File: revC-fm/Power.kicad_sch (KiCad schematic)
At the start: 55 parts, among them Q15 MMDT5551-7-F, Q16 MMDT5551-7-F, Q18 IRF7404TRPBF, Q32 MMBT4403WT1G, SW3 USB Charge Inhibit, SW4 High Inhibit, SW5 High USB Inhibit, SW6 Low Inhibit, U18 TPS54226PWPRPWP14_2P31X2P46-L, U19 ADM1176-1ARMZ-R7, U20 ADM1176-1ARMZ-R7, U21 BQ25883RGER

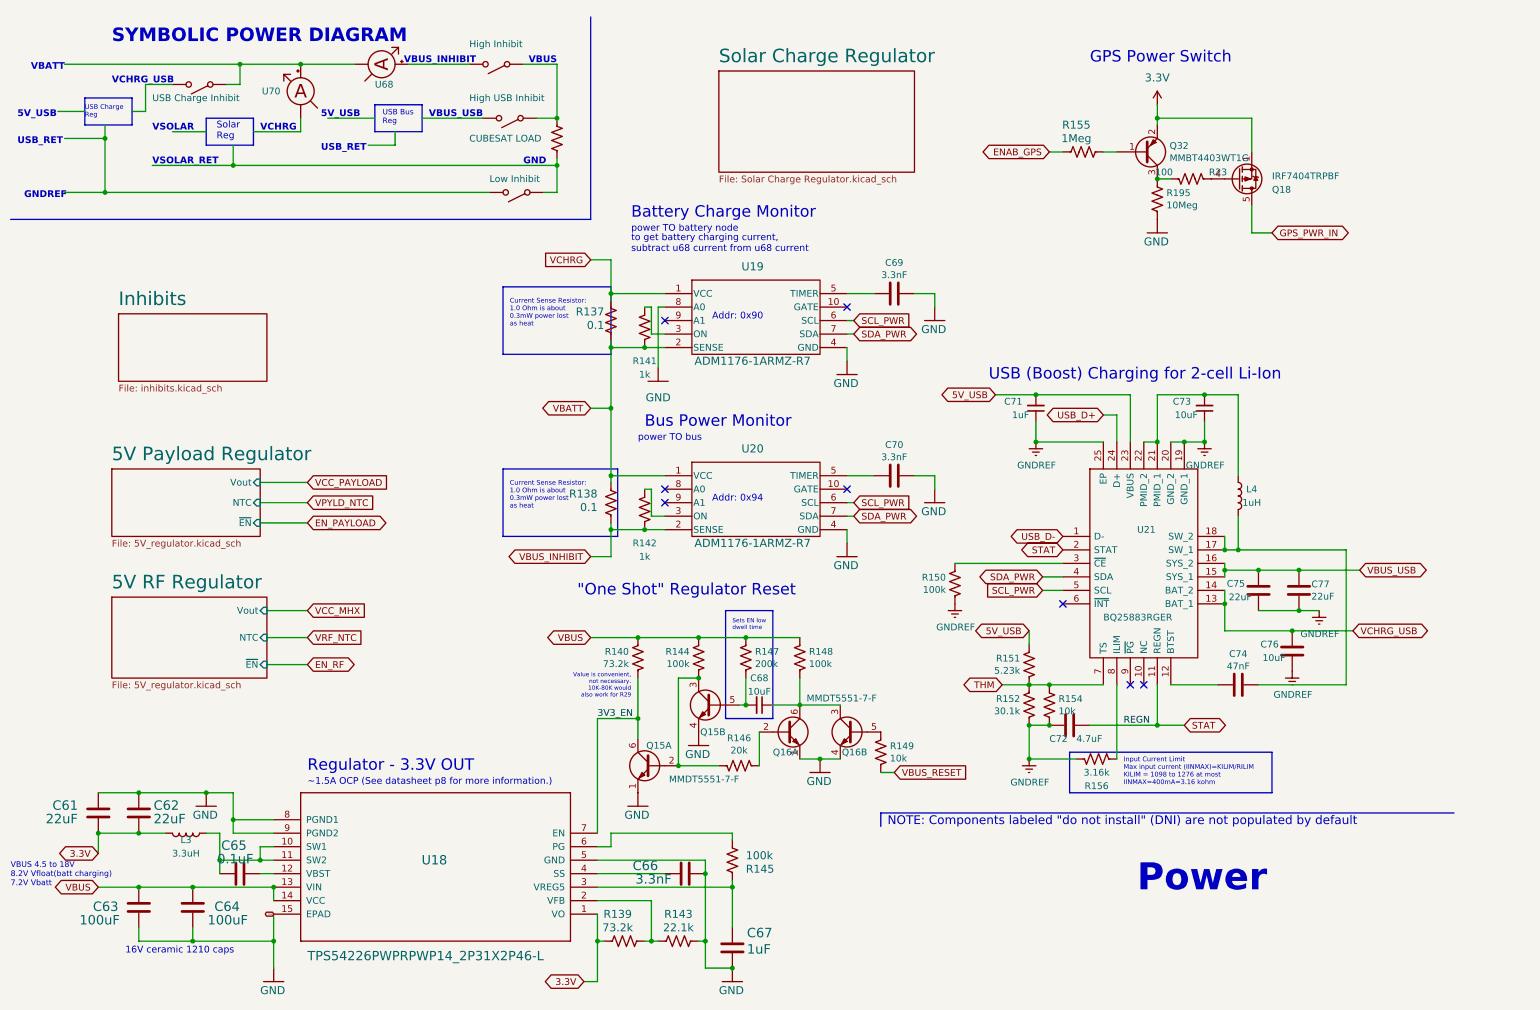
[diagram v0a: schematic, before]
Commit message: working revC
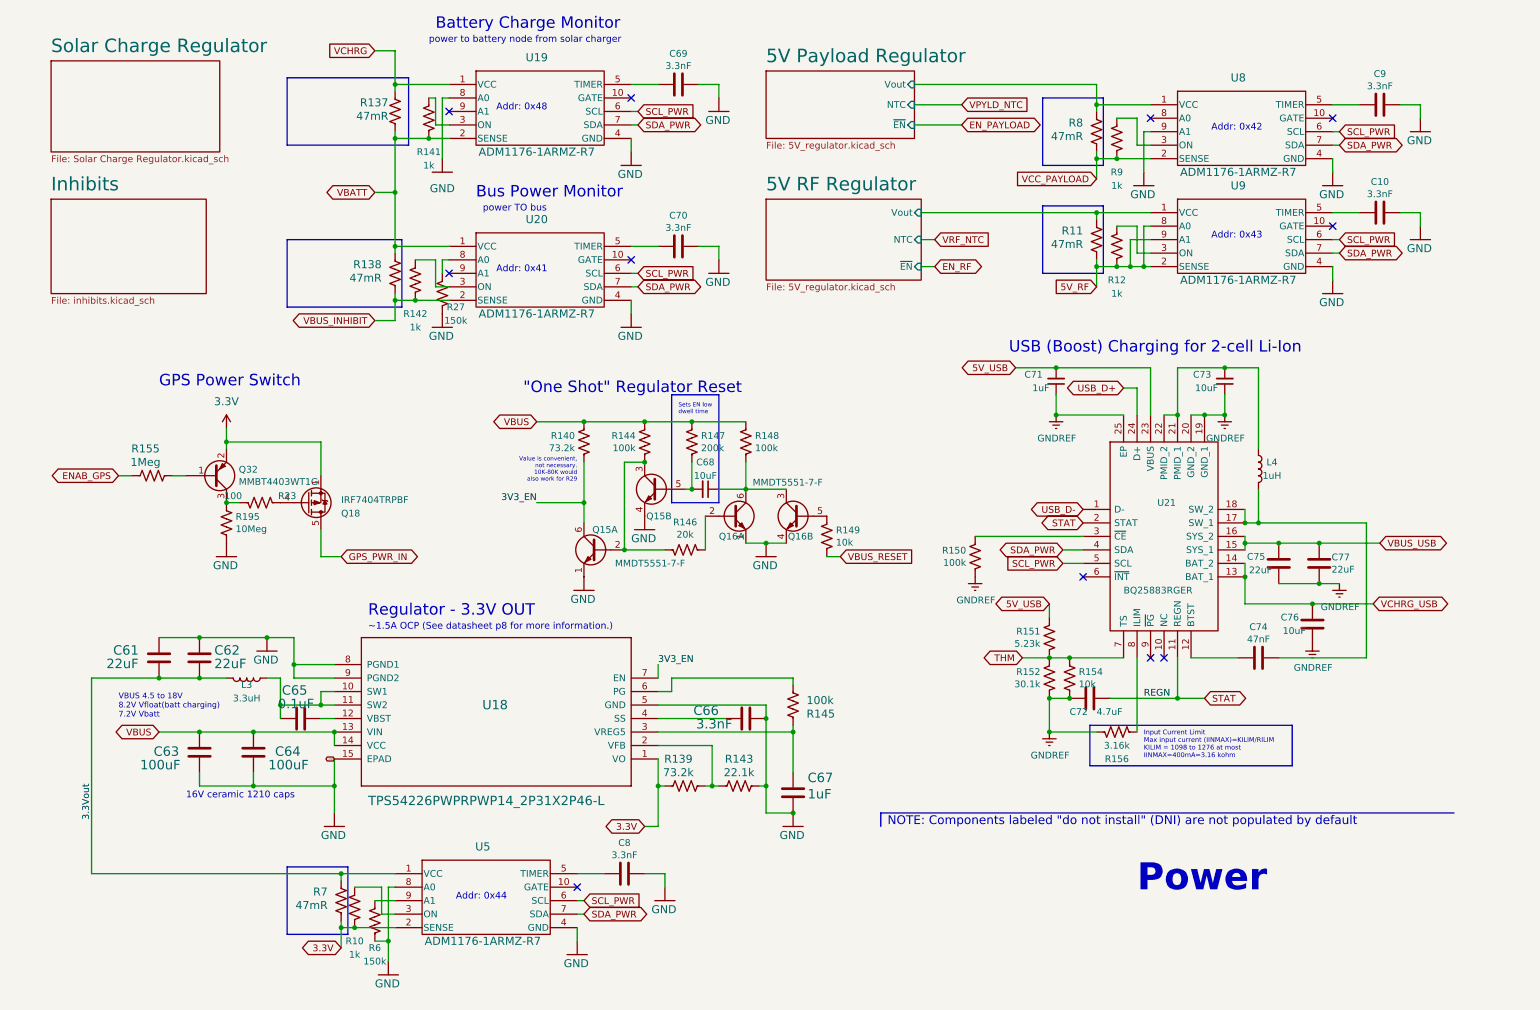
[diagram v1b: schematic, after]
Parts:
- removed MES1: U70, symbol Device:Ammeter_DC
- removed MES2: U68, symbol Device:Ammeter_DC
- removed R136: CUBESAT LOAD, symbol Device:R_US
- removed SW3: USB Charge Inhibit, symbol Switch:SW_SPST
- removed SW4: High Inhibit, symbol Switch:SW_SPST
- removed SW5: High USB Inhibit, symbol Switch:SW_SPST
- removed SW6: Low Inhibit, symbol Switch:SW_SPST
- added C10, C8, C9: 3.3nF, Capacitor_SMD:C_0603_1608Metric, symbol Device:C
- added R10, R12, R9: 1k, Resistor_SMD:R_0603_1608Metric, symbol Device:R_US
- added R11, R7, R8: 47mR, mainboard-SLI:KRL3216, symbol Device:R_US
- added R27, R6: 150k, Resistor_SMD:R_0603_1608Metric, symbol Device:R_US
- added U5, U8, U9: ADM1176-1ARMZ-R7, mainboard:ADM1176-1ARMZ-R7, symbol mainboard:ADM1176-1ARMZ-R7
- R137, R138: value 0.1 -> 47mR; footprint Resistor_SMD:R_2512_6332Metric -> mainboard-SLI:KRL3216
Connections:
- net 3.3V: now also R10.1, R7.1, U5.2 (SENSE); no longer C61.2, C62.2, L3.2
- net GND: now also C10.1, C8.1, C9.1, R27.1, R6.1, U5.4 (GND), U5.8 (A0), U8.4 (GND), U8.9 (A1), U9.4 (GND)
- net SCL_PWR: now also U5.6 (SCL), U8.6 (SCL), U9.6 (SCL)
- net SDA_PWR: now also U5.7 (SDA), U8.7 (SDA), U9.7 (SDA)
- net VCC_PAYLOAD: now also R8.1, R9.1, U8.2 (SENSE)
- net at U20.8 (A0): now also R27.2
- new net: R9.2, U8.3 (ON)
- new net: C9.2, U8.5 (TIMER)
- new net: R12.2, U9.3 (ON)
- new net: C10.2, U9.5 (TIMER)
- new net: R10.2, U5.3 (ON)
- new net: R6.2, U5.9 (A1)
- new net: C8.2, U5.5 (TIMER)
- new net 3.3Vout: C61.2, C62.2, L3.2, R7.2, U5.1 (VCC)
- new net 5V Payload Regulator/Vout: R8.2, U8.1 (VCC)
- new net 5V RF Regulator/Vout: R11.2, U9.1 (VCC)
- new net 5V_RF: R11.1, R12.1, U9.2 (SENSE), U9.8 (A0), U9.9 (A1)
- no-connect marks 8 -> 11
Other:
- note added: "Addr: 0x41"
- note added: "Addr: 0x42"
- note added: "Addr: 0x43"
- note added: "Addr: 0x44"
- note added: "Addr: 0x48"
- note added: "power to battery node from solar charger"
- note removed: "5V_USB"
- note removed: "Addr: 0x90"
- note removed: "Addr: 0x94"
- note removed: "Current Sense Resistor: 1.0 Ohm is about 0.3mW power lost as heat"
- note removed: "GND"
- note removed: "GNDREF"
- note removed: "SYMBOLIC POWER DIAGRAM"
- note removed: "Solar Reg"
- note removed: "USB Bus Reg"
- note removed: "USB Charge Reg"
- note removed: "USB_RET"
- note removed: "VBATT"
- note removed: "VBUS"
- note removed: "VBUS_INHIBIT"
- note removed: "VBUS_USB"
- note removed: "VCHRG"
- note removed: "VCHRG_USB"
- note removed: "VSOLAR"
- note removed: "VSOLAR_RET"
- note removed: "power TO battery node"
- note removed: "to get battery charging current, subtract u68 current from u68 current"
- moved on the sheet: C61, C62, C63, C64, C65, C66, C67, C68, C69, C70, C71, C72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
